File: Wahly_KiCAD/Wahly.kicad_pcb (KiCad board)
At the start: 2 copper layers, 50.1 x 50.1 mm, 46 parts, among them J1 USB_B_Micro, J2 Power, J3 ADC, J4 SWD, J5 TIM2, SW1 SW_SPDT, U1 LM1117-3.3, U2 USBLC6-2SC6, U3 SHT30-DIS, U4 LIS3DHTR, U5 STM32F302C8Tx, U6 W25Q32JVSS, Y1 16MHz

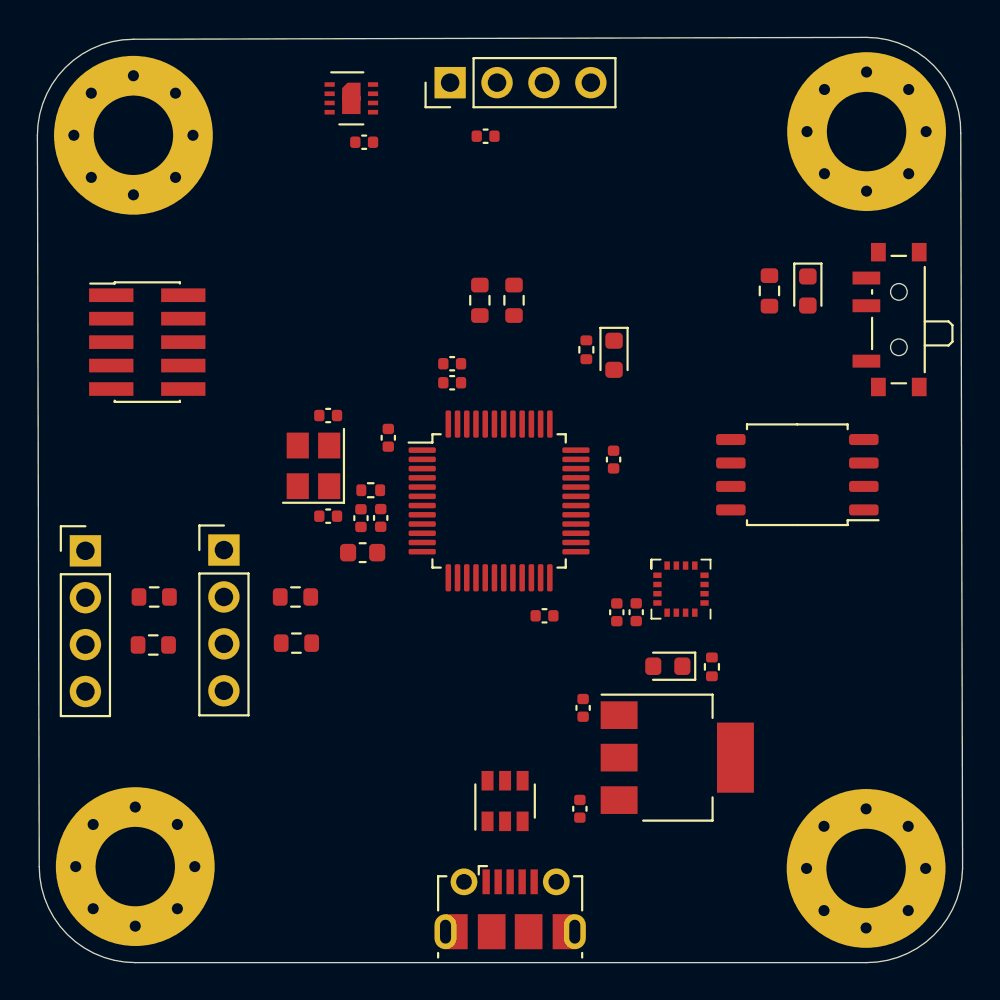
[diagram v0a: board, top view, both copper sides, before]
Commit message: Silkscreen & DRC
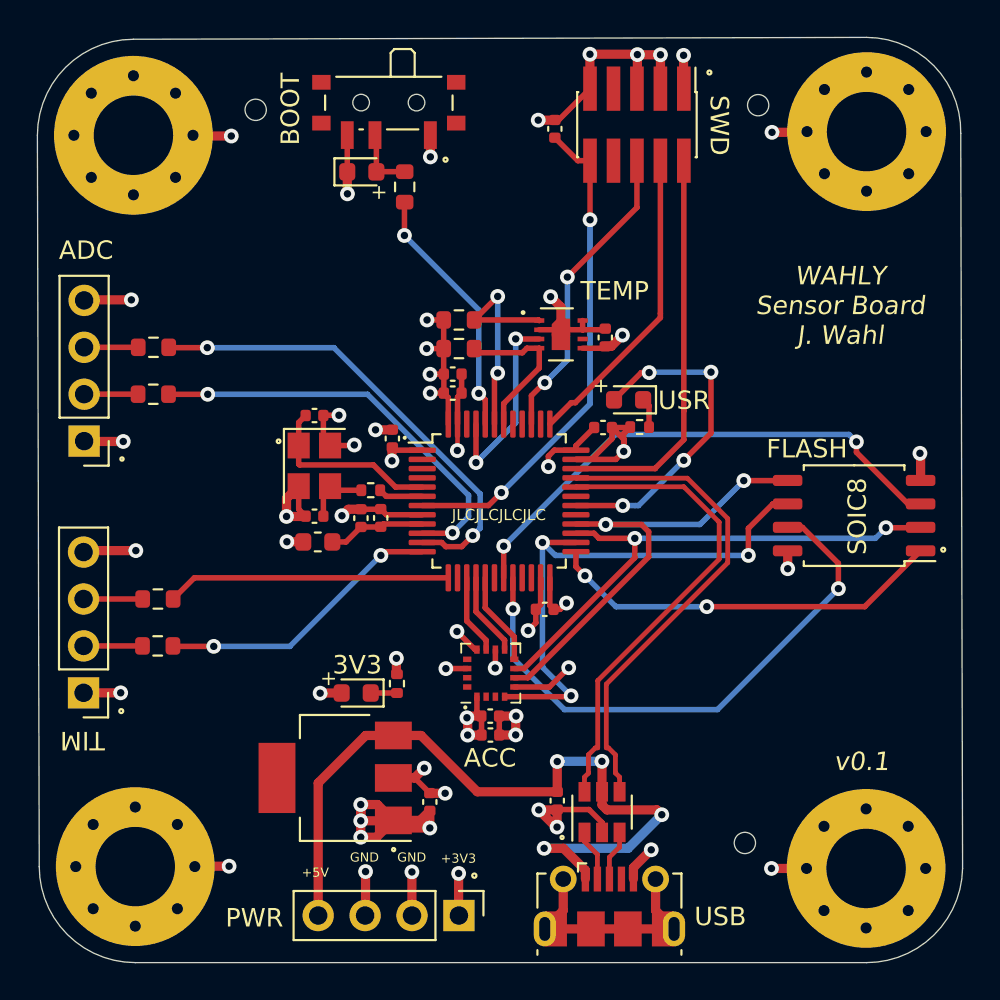
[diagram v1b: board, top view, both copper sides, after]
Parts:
- moved J2 45.1 mm to (72.3, 111.5), turned to 270 degrees
- moved SW1 29.6 mm to (68.5, 67.9), turned to 180 degrees
- moved J4 29.0 mm to (82.0, 68.7), turned to 270 degrees
- moved D4 25.0 mm to (67.1, 71.3), turned to 0 degrees
- moved R9 20.5 mm to (69.4, 72.1), turned to 270 degrees
- moved U1 18.6 mm to (65.6, 104.1), turned to 180 degrees
- moved U3 17.1 mm to (77.8, 80.1)
- moved R4 17.1 mm to (69.0, 99.0), turned to 90 degrees
- moved D1 16.9 mm to (66.8, 99.5)
- moved C3 16.8 mm to (80.2, 80.2), turned to 90 degrees
- moved R7 16.1 mm to (55.8, 80.8)
- moved U4 11.3 mm to (74.0, 98.4), turned to 90 degrees
- moved R6 11.0 mm to (55.8, 83.3)
- moved J5 10.8 mm to (52.0, 99.5), turned to 180 degrees
- moved C2 9.74 mm to (70.8, 105.4), turned to 270 degrees
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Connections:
- J4 pad 6: SWD_DIO -> SWD_SWO
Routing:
- net GND: track 0.00 -> 119.6 mm, vias 0 -> 36
- net +3V3: track 0.00 -> 43.7 mm, vias 0 -> 21
- net +5V: track 0.00 -> 42.7 mm, vias 0 -> 4
- net FLASH_!HOLD: track 0.00 -> 30.8 mm, vias 0 -> 2
- net SPI2_SCK: track 0.00 -> 30.0 mm, vias 0 -> 3
- net SPI2_MISO: track 0.00 -> 29.1 mm, vias 0 -> 2
- net FLASH_!WP: track 0.00 -> 28.7 mm, vias 0 -> 2
- net USB_D+: track 0.00 -> 27.0 mm
- net NRST: track 0.00 -> 27.0 mm, vias 0 -> 2
- net SPI2_MOSI: track 0.00 -> 26.3 mm, vias 0 -> 2
- net USB_D-: track 0.00 -> 26.3 mm
- net ADC1_IN2: track 0.00 -> 25.7 mm, vias 0 -> 2
- net ADC1_IN1: track 0.00 -> 22.6 mm, vias 0 -> 2
- net SPI2_!CS: track 0.00 -> 21.6 mm, vias 0 -> 2
- net SWD_DIO: track 0.00 -> 21.6 mm
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- added copper zone on In2.Cu, net +3V3
- added copper zone on In1.Cu, net GND
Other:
- outline, holes or cut-outs redrawn
- copper layers 2 -> 4
- board text added: "+"
- board text added: "+3V3"
- board text added: "+5V"
- board text added: "3V3"
- board text added: "ACC"
- board text added: "ADC"
- board text added: "BOOT"
- board text added: "FLASH"
- board text added: "GND"
- board text added: "JLCJLCJLCJLC"
- board text added: "PWR"
- board text added: "SOIC8"
- board text added: "SWD"
- board text added: "TEMP"
- board text added: "TIM"
- board text added: "USB"
- board text added: "USR"
- board text added: "WAHLY Sensor Board J. Wahl"
- board text added: "v0.1"
